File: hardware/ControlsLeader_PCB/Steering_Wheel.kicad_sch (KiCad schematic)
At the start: 4 parts, among them J10 Indicator_Switch, Q6 NMOS

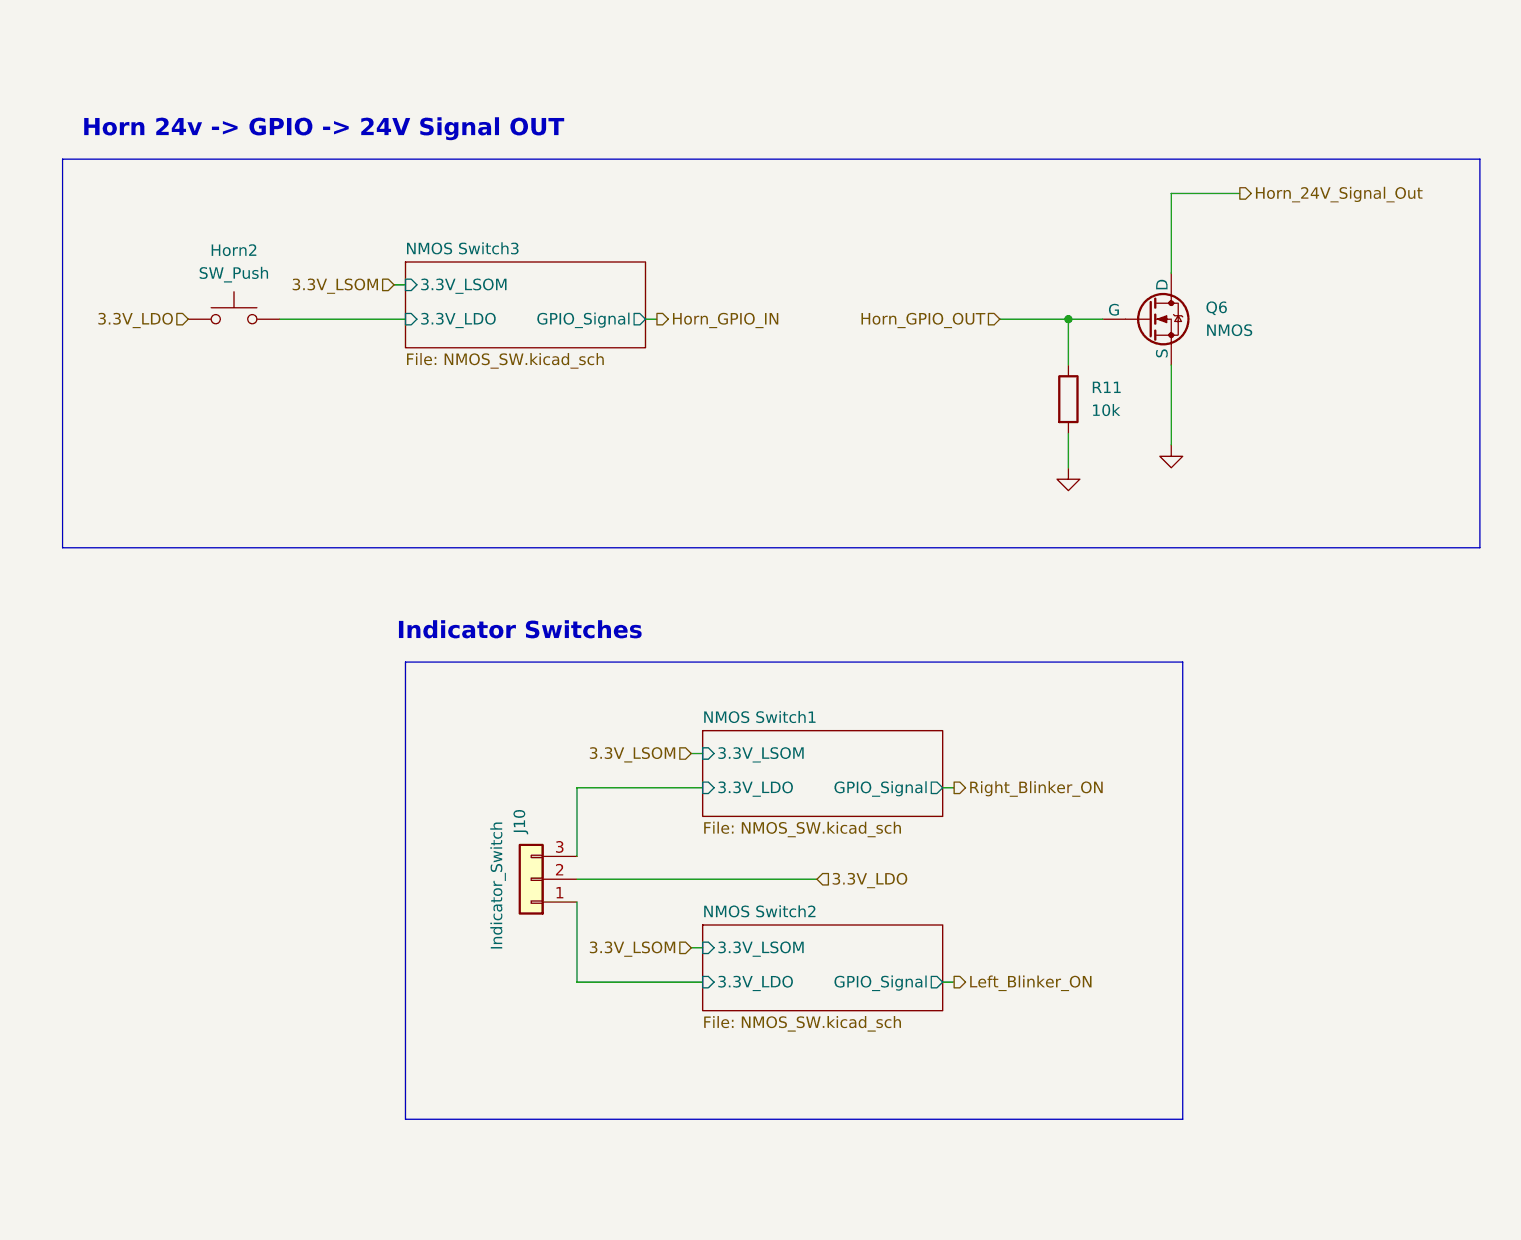
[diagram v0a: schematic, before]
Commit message: Ready for final review
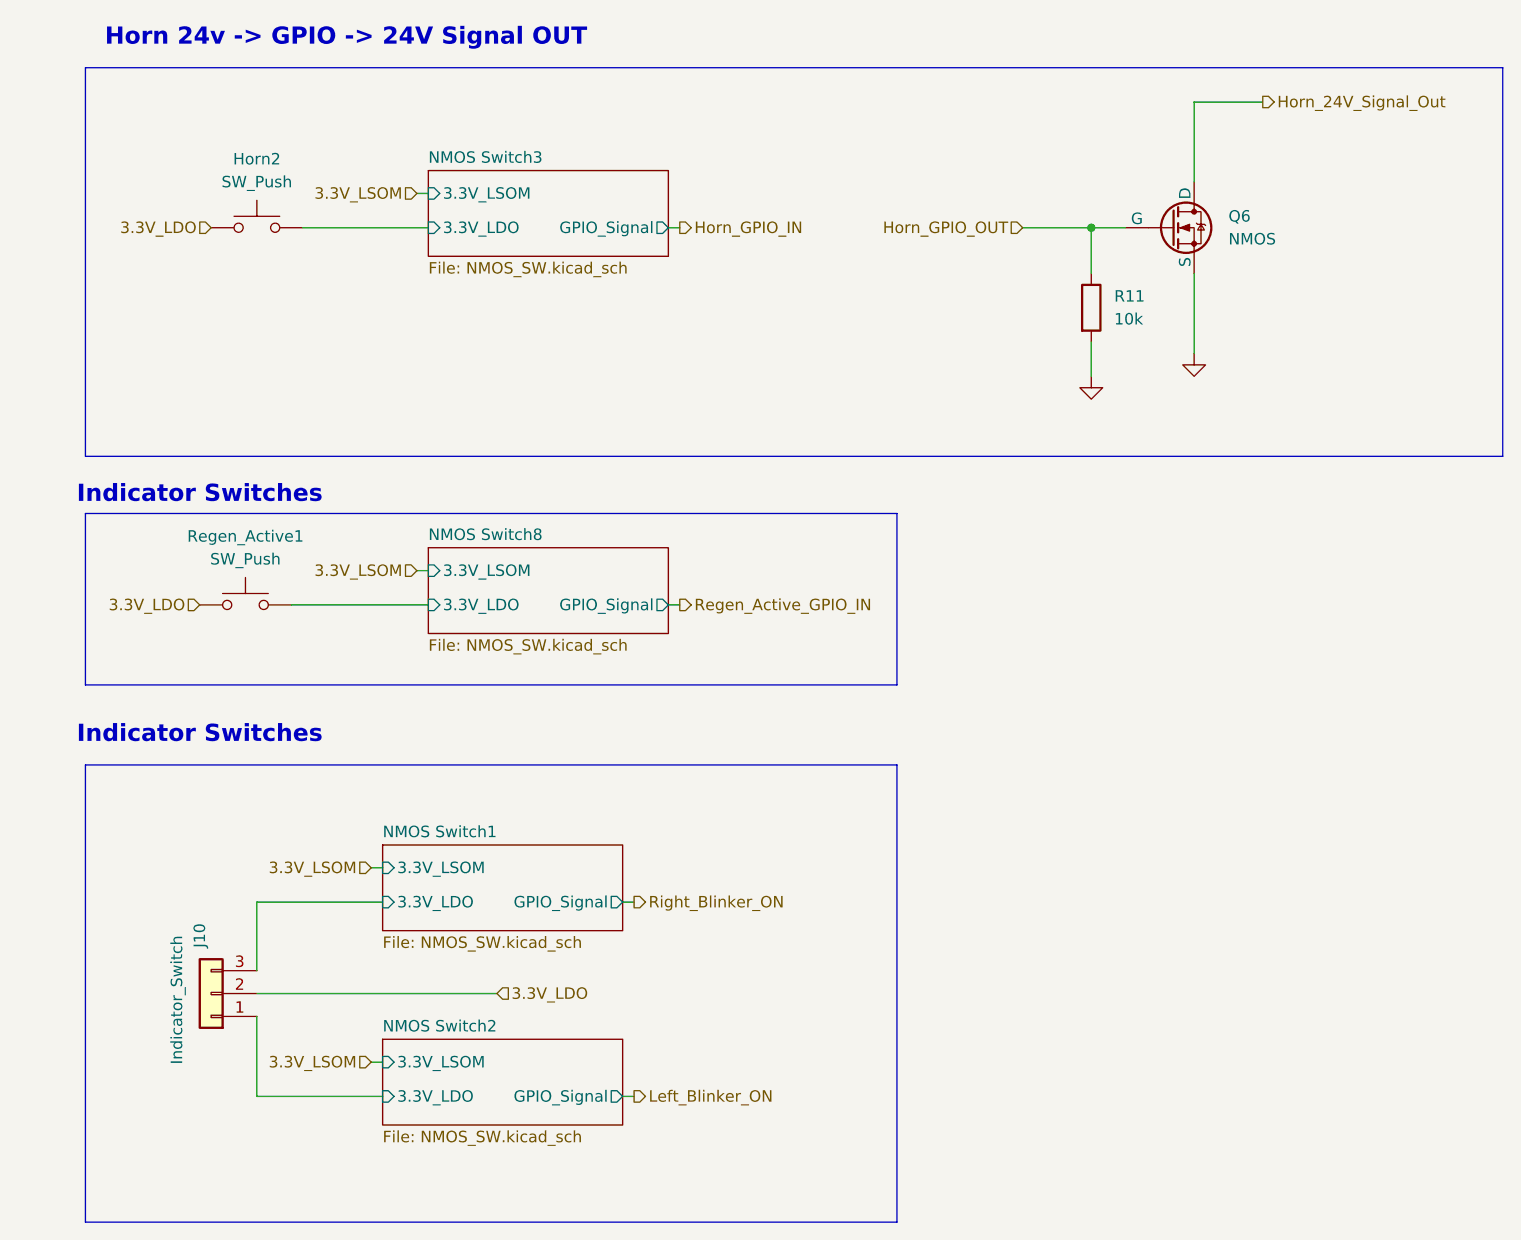
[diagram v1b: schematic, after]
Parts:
- added Regen_Active1: SW_Push, Connector_Molex:Molex_Nano-Fit_105313-xx02_1x02_P2.50mm_Horizontal, symbol Switch:SW_Push
- Horn2: Distributor Link (none) -> https://www.amazon.com/Gebildet-Waterproof-Momentary-Lockle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; Manufacturer (none) -> Amazon
- J10: footprint Connector_Molex:Molex_Micro-Fit_3.0_43650-0300_1x03_P3.00mm_Horizontal -> Connector_Molex:Molex_Nano-Fit_105313-xx03_1x03_P2.50mm_Horizontal; Distributor Link (none) -> https://www.amazon.com/XINYIELE-Rocker-Switch-Position-Circ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; Manufacturer (none) -> Amazon
- Q6: footprint (none) -> LSOM_IRLM:SOT23
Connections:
- net 3.3V_LDO: now also Regen_Active1.1
- new net NMOS Switch8/3.3V_LDO: Regen_Active1.2
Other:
- added sheet NMOS Switch8 (NMOS_SW.kicad_sch)
- moved on the sheet: Horn2, J10, Q6, R11
